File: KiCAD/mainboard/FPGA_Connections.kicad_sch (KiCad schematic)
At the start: 1 part, among them J100 AHDF15A-KG-TAXB

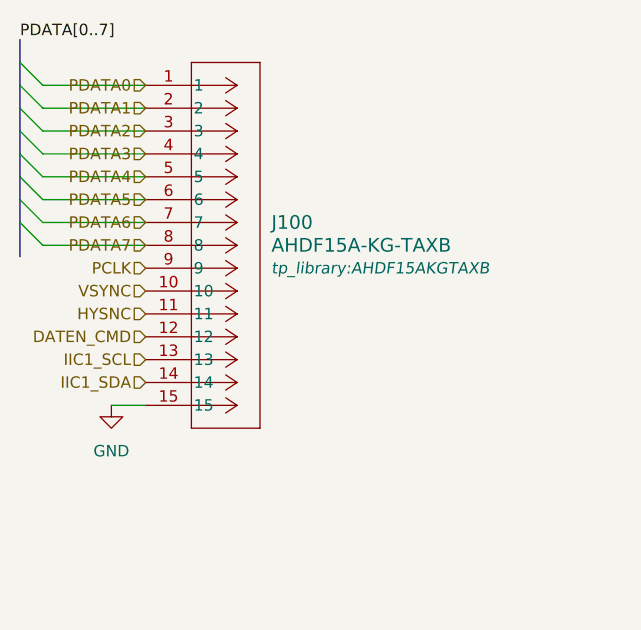
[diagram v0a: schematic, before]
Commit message: refactor
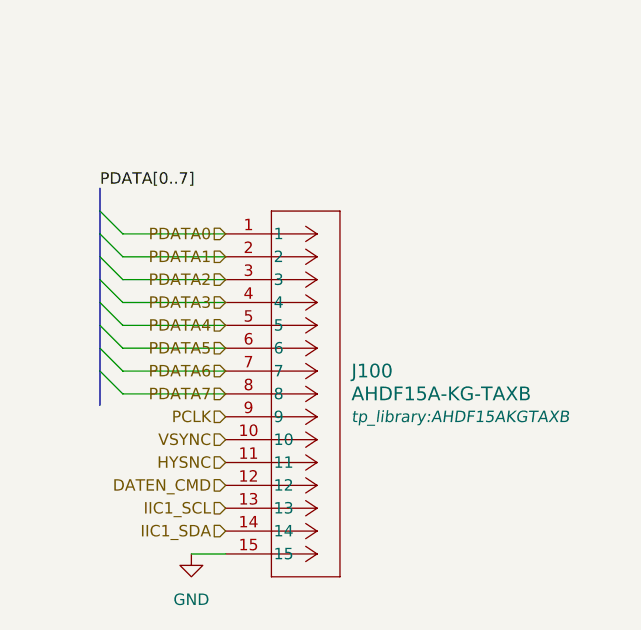
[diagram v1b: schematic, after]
